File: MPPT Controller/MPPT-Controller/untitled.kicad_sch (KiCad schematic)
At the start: 29 parts, among them J5 USB_C_Receptacle_USB2.0_16P, U2 ESP32-WROOM-32D, U3 CH340C

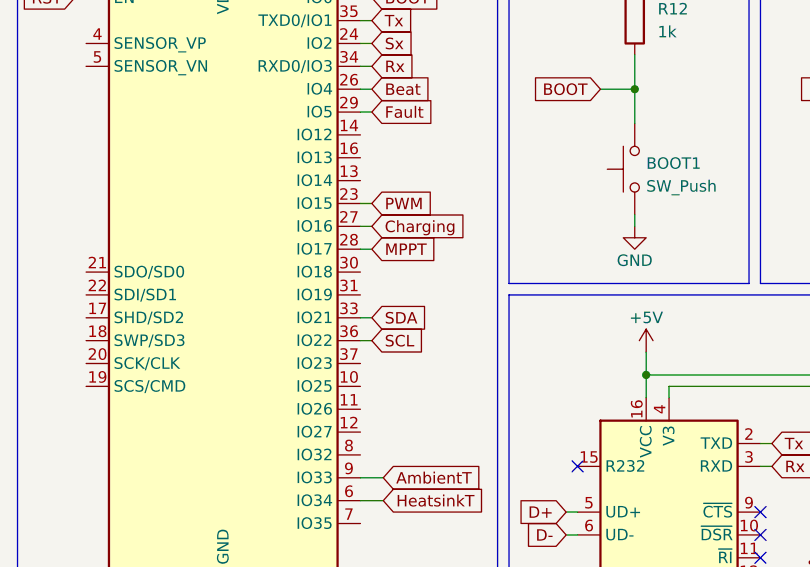
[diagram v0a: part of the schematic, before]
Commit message: Diode
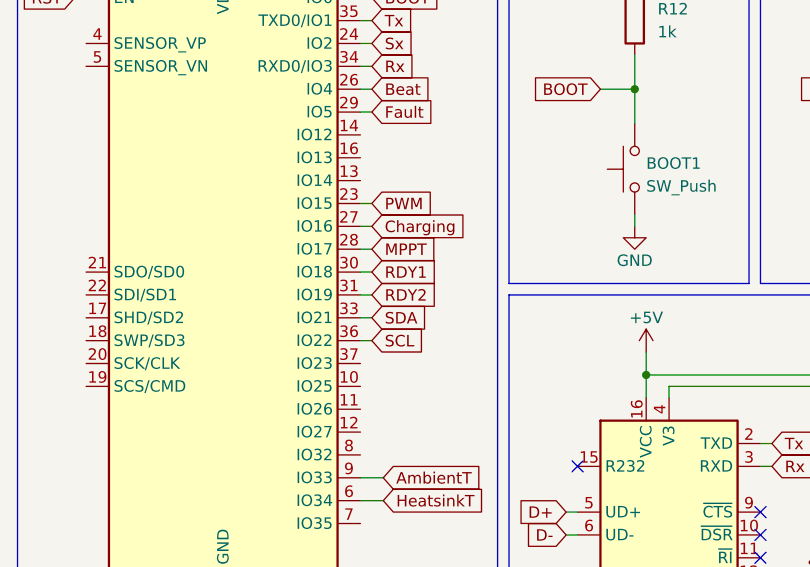
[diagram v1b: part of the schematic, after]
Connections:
- net RDY1: now reaches U2.30 (IO18)
- net RDY2: now reaches U2.31 (IO19)
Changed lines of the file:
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@@
+	(wire
+		(pts
+			(xy 50.8 58.42) (xy 52.07 58.42)
+		)
+		(stroke
+			(width 0)
+			(type default)
+		)
+	)
 	(wire
 		(pts
@@
 	(wire
 		(pts
+			(xy 50.8 55.88) (xy 52.07 55.88)
+		)
+		(stroke
+			(width 0)
+			(type default)
+		)
+	)
+	(wire
+		(pts
 			(xy 38.1 139.7) (xy 38.1 143.51)
 		)
@@
 		)
 	)
+	(global_label "RDY1"
+		(shape input)
+		(at 52.07 55.88 0)
+		(fields_autoplaced yes)
+		(effects
+			(font
+				(size 1.27 1.27)
+			)
+			(justify left)
+		)
+		(property "Intersheetrefs" "${INTERSHEET_REFS}"
+			(at 59.8933 55.88 0)
+			(effects
+				(font
+					(size 1.27 1.27)
+				)
+				(justify left)
+				(hide yes)
+			)
+		)
+	)
 	(global_label "Rx"
 		(shape input)
@@
 			(effects
 				(font
+					(size 1.27 1.27)
+				)
+				(justify left)
+				(hide yes)
+			)
+		)
+	)
+	(global_label "RDY2"
+		(shape input)
+		(at 52.07 58.42 0)
+		(fields_autoplaced yes)
+		(effects
+			(font
+				(size 1.27 1.27)
+			)
+			(justify left)
+		)
+		(property "Intersheetrefs" "${INTERSHEET_REFS}"
+			(at 59.8933 58.42 0)
+			(effects
+				(font
